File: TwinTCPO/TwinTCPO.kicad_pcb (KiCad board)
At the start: 2 copper layers, 82.3 x 42.7 mm, 44 parts, among them J1 Power In, J2 Key In, J3 Spk, J4 Phone, Q1 2N4401, Q2 2N7000, Q3 2N4401, Q4 2N4401, Q5 2N4403, U1 LM386

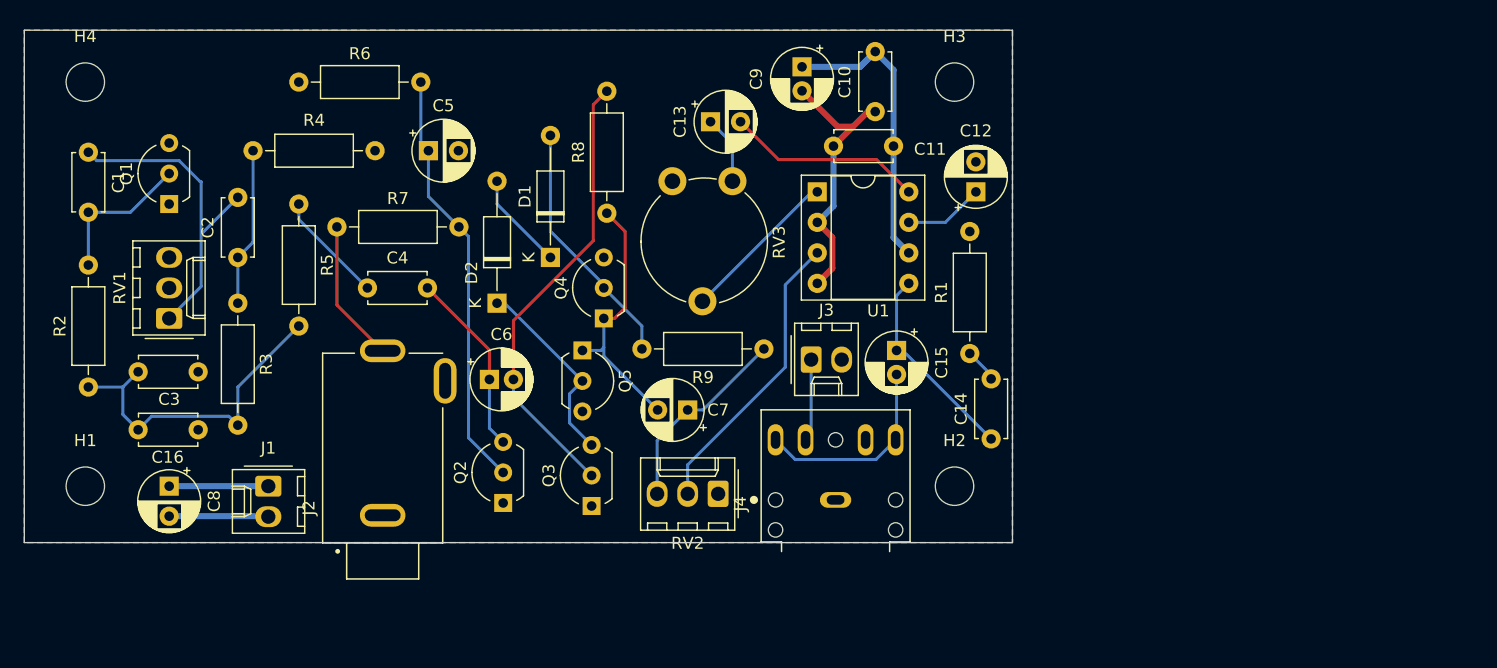
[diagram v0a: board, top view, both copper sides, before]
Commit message: Ready for production
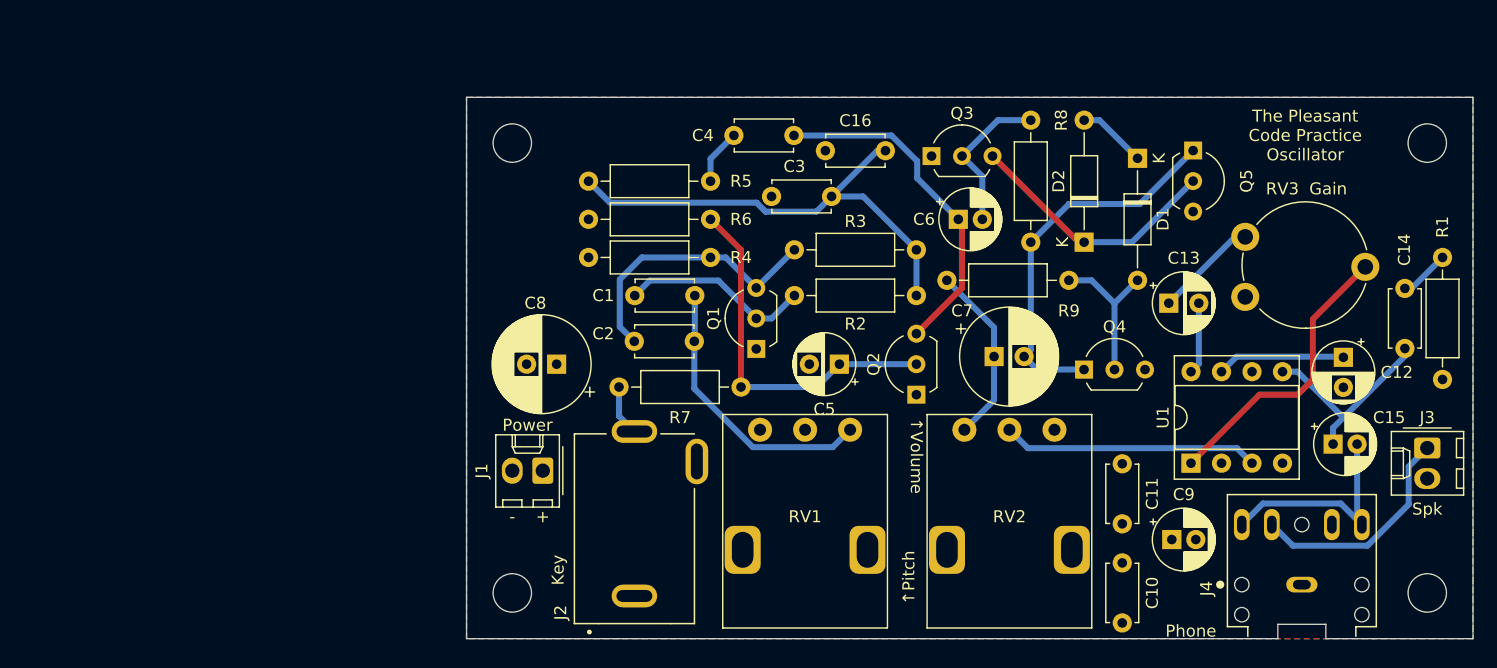
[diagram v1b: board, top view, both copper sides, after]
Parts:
- C7, C8: footprint Capacitor_THT:CP_Radial_D5.0mm_P2.50mm -> Capacitor_THT:CP_Radial_D8.0mm_P2.50mm
- J1: value Power In -> Power
- J2: value Key In -> Key
- RV1, RV2: footprint Connector_Molex:Molex_KK-254_AE-6410-03A_1x03_P2.54mm_Vertical -> MyLibrary:P120PK
- moved H4 119.6 mm to (137.2, 128.9)
- moved R2 69.4 mm to (94.6, 104.1), turned to 180 degrees
- moved C16 57.2 mm to (87.0, 92.1), turned to 0 degrees
- moved RV1 53.8 mm to (85.3, 115.3), turned to 180 degrees
- moved Q5 53.5 mm to (117.7, 92.1)
- moved C1 51.9 mm to (76.2, 104.1), turned to 180 degrees
- moved J3 51.8 mm to (137.2, 116.8), turned to -90 degrees
- moved Q1 50.4 mm to (81.3, 108.6)
- moved C9 50.0 mm to (115.9, 124.5), turned to 0 degrees
- moved C3 49.9 mm to (82.5, 95.9), turned to 0 degrees
- moved D1 49.6 mm to (113.0, 92.7), turned to -90 degrees
- moved D2 49.2 mm to (108.6, 99.7)
- moved RV3 48.7 mm to (122.0, 104.3), turned to 0 degrees
- moved C10 47.3 mm to (111.8, 126.4)
- moved R3 46.6 mm to (84.5, 100.3), turned to 0 degrees
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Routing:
- net VCC: track 34.6 -> 0.00 mm
- net GND: track 31.4 -> 0.00 mm
- net Net-(C6-Pad2): track 37.9 -> 12.9 mm
- net Net-(C4-Pad2): track 15.4 -> 28.6 mm
- net Net-(C16-Pad2): track 28.2 -> 40.6 mm
- net Net-(J3-Pad1): track 6.88 -> 18.9 mm
- net Net-(RV3-Pad2): track 13.3 -> 24.2 mm
- net Net-(C13-Pad2): track 16.4 -> 5.97 mm
- net Net-(C2-Pad1): track 13.2 -> 23.3 mm
- net Net-(C7-Pad2): track 22.0 -> 31.9 mm
- net Net-(D1-Pad2): track 20.9 -> 12.8 mm
- net Net-(J2-Pad2): track 11.9 -> 4.23 mm
- net Net-(C5-Pad1): track 35.4 -> 30.4 mm
- net Net-(D2-Pad1): track 17.0 -> 21.8 mm
- net Net-(C4-Pad1): track 9.35 -> 4.62 mm
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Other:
- board size 82.3 x 42.7 mm -> 83.8 x 45.1 mm
- net class Default removed
- board text added: "+"
- board text added: "-"
- board text added: "Gain"
- board text added: "JLCJLCJLCJLC"
- board text added: "Key"
- board text added: "Layout by M. McLure WW1FA Based on work by M. Maynard K4ICY and S. Smith G0TDJ"
- board text added: "Phone"
- board text added: "Power"
- board text added: "Spk"
- board text added: "The Pleasant Code Practice Oscillator"
- board text added: "↑Pitch"
- board text added: "↑Volume"
